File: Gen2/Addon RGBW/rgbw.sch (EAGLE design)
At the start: 33 parts, among them Q1 BUZ11, Q2 BUZ11, Q3 BUZ11, Q4 BUZ11, Q5 BUZ11, Q6 BUZ11, Q7 BUZ11, Q8 BUZ11

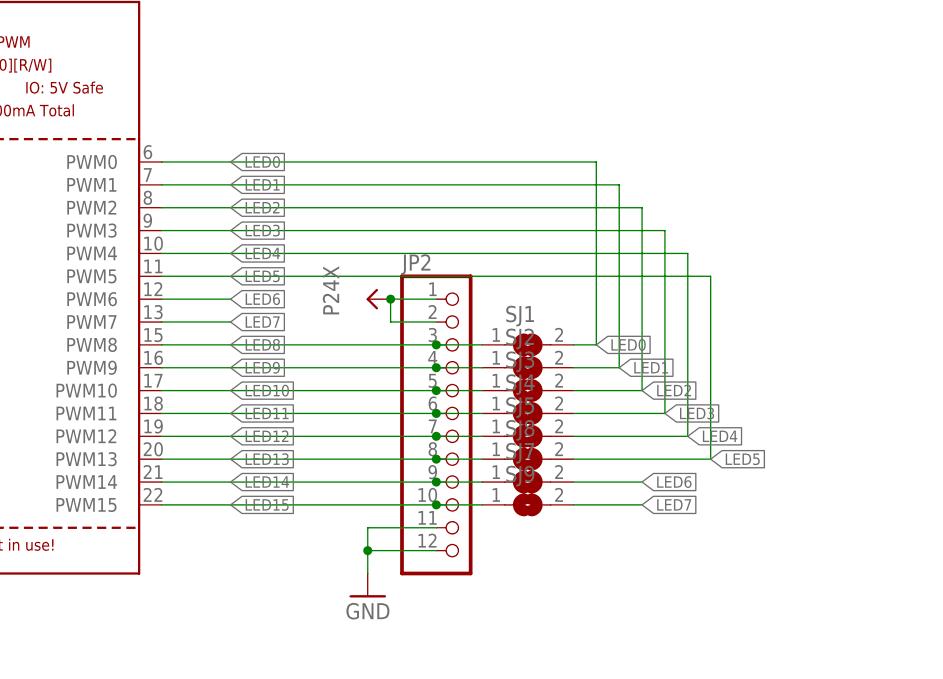
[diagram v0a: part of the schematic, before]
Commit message: ordner umsortiert und module weiter gemacht
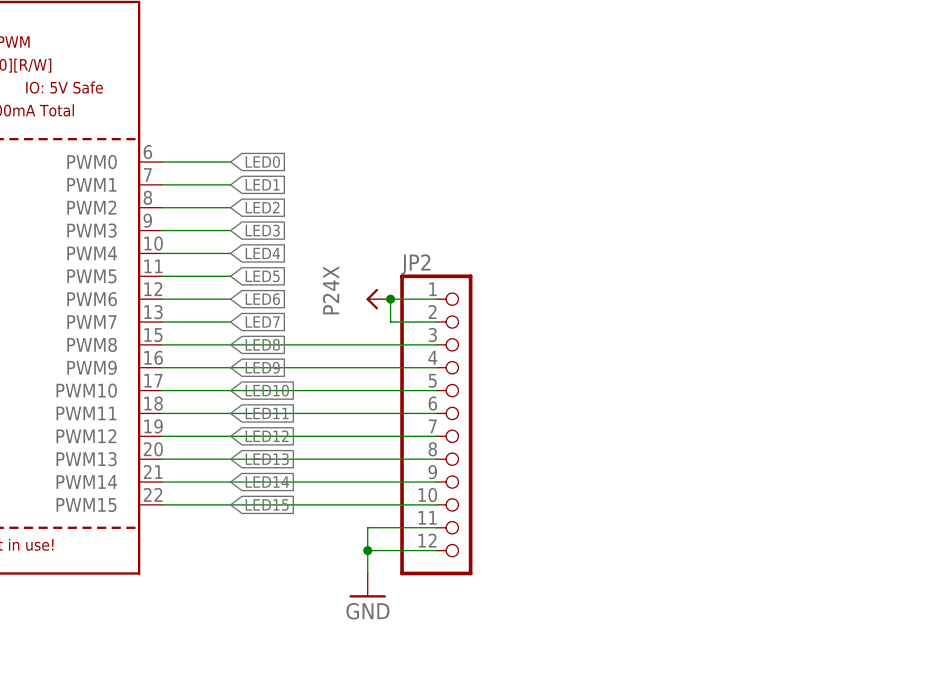
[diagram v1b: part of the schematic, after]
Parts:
- removed SJ1, SJ2, SJ3, SJ4, SJ5, SJ7, SJ8, SJ9: (no value), jumper:SJ
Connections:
- net LED0: no longer SJ1.2
- net LED1: no longer SJ2.2
- net LED10: no longer SJ3.1
- net LED11: no longer SJ4.1
- net LED12: no longer SJ5.1
- net LED13: no longer SJ8.1
- net LED14: no longer SJ7.1
- net LED15: no longer SJ9.1
- net LED2: no longer SJ3.2
- net LED3: no longer SJ4.2
- net LED4: no longer SJ5.2
- net LED5: no longer SJ8.2
- net LED6: no longer SJ7.2
- net LED7: no longer SJ9.2
- net LED8: no longer SJ1.1
- net LED9: no longer SJ2.1
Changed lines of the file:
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@@
 <part name="SUPPLY9" library="schlager_supply" deviceset="P24X" device=""/>
 <part name="GND12" library="supply1" deviceset="GND" device=""/>
-<part name="SJ1" library="jumper" deviceset="SJ" device=""/>
-<part name="SJ2" library="jumper" deviceset="SJ" device=""/>
-<part name="SJ3" library="jumper" deviceset="SJ" device=""/>
-<part name="SJ4" library="jumper" deviceset="SJ" device=""/>
-<part name="SJ5" library="jumper" deviceset="SJ" device=""/>
-<part name="SJ7" library="jumper" deviceset="SJ" device=""/>
-<part name="SJ8" library="jumper" deviceset="SJ" device=""/>
-<part name="SJ9" library="jumper" deviceset="SJ" device=""/>
 </parts>
 <sheets>
@@
 <instance part="SUPPLY9" gate="G$1" x="152.4" y="114.3" rot="R90"/>
 <instance part="GND12" gate="1" x="152.4" y="81.28" rot="MR0"/>
-<instance part="SJ1" gate="1" x="170.18" y="109.22"/>
-<instance part="SJ2" gate="1" x="170.18" y="106.68"/>
-<instance part="SJ3" gate="1" x="170.18" y="104.14"/>
-<instance part="SJ4" gate="1" x="170.18" y="101.6"/>
-<instance part="SJ5" gate="1" x="170.18" y="99.06"/>
-<instance part="SJ7" gate="1" x="170.18" y="93.98"/>
-<instance part="SJ8" gate="1" x="170.18" y="96.52"/>
-<instance part="SJ9" gate="1" x="170.18" y="91.44"/>
 </instances>
 <busses>
@@
 <pinref part="U1" gate="G$1" pin="PWM4"/>
 <label x="137.16" y="119.38" size="1.27" layer="95" xref="yes"/>
-<wire x1="129.54" y1="119.38" x2="187.96" y2="119.38" width="0.1524" layer="91"/>
-<wire x1="187.96" y1="119.38" x2="187.96" y2="99.06" width="0.1524" layer="91"/>
-<pinref part="SJ5" gate="1" pin="2"/>
-<wire x1="187.96" y1="99.06" x2="175.26" y2="99.06" width="0.1524" layer="91"/>
-<label x="187.96" y="99.06" size="1.27" layer="95" xref="yes"/>
+<wire x1="129.54" y1="119.38" x2="137.16" y2="119.38" width="0.1524" layer="91"/>
 </segment>
 </net>
@@
 <pinref part="U1" gate="G$1" pin="PWM5"/>
 <label x="137.16" y="116.84" size="1.27" layer="95" xref="yes"/>
-<wire x1="129.54" y1="116.84" x2="190.5" y2="116.84" width="0.1524" layer="91"/>
-<wire x1="190.5" y1="116.84" x2="190.5" y2="96.52" width="0.1524" layer="91"/>
-<pinref part="SJ8" gate="1" pin="2"/>
-<wire x1="190.5" y1="96.52" x2="175.26" y2="96.52" width="0.1524" layer="91"/>
-<label x="190.5" y="96.52" size="1.27" layer="95" xref="yes"/>
+<wire x1="129.54" y1="116.84" x2="137.16" y2="116.84" width="0.1524" layer="91"/>
 </segment>
 </net>
@@
 <label x="137.16" y="114.3" size="1.27" layer="95" xref="yes"/>
 </segment>
-<segment>
-<pinref part="SJ7" gate="1" pin="2"/>
-<wire x1="175.26" y1="93.98" x2="182.88" y2="93.98" width="0.1524" layer="91"/>
-<label x="182.88" y="93.98" size="1.27" layer="95" xref="yes"/>
-</segment>
 </net>
 <net name="LED7" class="0">
@@
 <pinref part="U1" gate="G$1" pin="PWM7"/>
 <label x="137.16" y="111.76" size="1.27" layer="95" xref="yes"/>
-</segment>
-<segment>
-<pinref part="SJ9" gate="1" pin="2"/>
-<wire x1="182.88" y1="91.44" x2="175.26" y2="91.44" width="0.1524" layer="91"/>
-<label x="182.88" y="91.44" size="1.27" layer="95" xref="yes"/>
 </segment>
 </net>
@@
 <pinref part="U1" gate="G$1" pin="PWM0"/>
 <label x="137.16" y="129.54" size="1.27" layer="95" xref="yes"/>
-<pinref part="SJ1" gate="1" pin="2"/>
-<wire x1="175.26" y1="109.22" x2="177.8" y2="109.22" width="0.1524" layer="91"/>
-<wire x1="177.8" y1="109.22" x2="177.8" y2="129.54" width="0.1524" layer="91"/>
-<wire x1="177.8" y1="129.54" x2="129.54" y2="129.54" width="0.1524" layer="91"/>
-<label x="177.8" y="109.22" size="1.27" layer="95" xref="yes"/>
+<wire x1="137.16" y1="129.54" x2="129.54" y2="129.54" width="0.1524" layer="91"/>
 </segment>
 </net>
@@
 <pinref part="U1" gate="G$1" pin="PWM1"/>
 <label x="137.16" y="127" size="1.27" layer="95" xref="yes"/>
-<wire x1="129.54" y1="127" x2="180.34" y2="127" width="0.1524" layer="91"/>
-<wire x1="180.34" y1="127" x2="180.34" y2="106.68" width="0.1524" layer="91"/>
-<pinref part="SJ2" gate="1" pin="2"/>
-<wire x1="180.34" y1="106.68" x2="175.26" y2="106.68" width="0.1524" layer="91"/>
-<label x="180.34" y="106.68" size="1.27" layer="95" xref="yes"/>
+<wire x1="129.54" y1="127" x2="137.16" y2="127" width="0.1524" layer="91"/>
 </segment>
 </net>
@@
 <pinref part="U1" gate="G$1" pin="PWM2"/>
 <label x="137.16" y="124.46" size="1.27" layer="95" xref="yes"/>
-<wire x1="129.54" y1="124.46" x2="182.88" y2="124.46" width="0.1524" layer="91"/>
-<wire x1="182.88" y1="124.46" x2="182.88" y2="104.14" width="0.1524" layer="91"/>
-<pinref part="SJ3" gate="1" pin="2"/>
-<wire x1="182.88" y1="104.14" x2="175.26" y2="104.14" width="0.1524" layer="91"/>
-<label x="182.88" y="104.14" size="1.27" layer="95" xref="yes"/>
+<wire x1="129.54" y1="124.46" x2="137.16" y2="124.46" width="0.1524" layer="91"/>
 </segment>
 </net>
@@
 <pinref part="U1" gate="G$1" pin="PWM3"/>
 <label x="137.16" y="121.92" size="1.27" layer="95" xref="yes"/>
-<wire x1="129.54" y1="121.92" x2="185.42" y2="121.92" width="0.1524" layer="91"/>
-<wire x1="185.42" y1="121.92" x2="185.42" y2="101.6" width="0.1524" layer="91"/>
-<pinref part="SJ4" gate="1" pin="2"/>
-<wire x1="185.42" y1="101.6" x2="175.26" y2="101.6" width="0.1524" layer="91"/>
-<label x="185.42" y="101.6" size="1.27" layer="95" xref="yes"/>
+<wire x1="129.54" y1="121.92" x2="137.16" y2="121.92" width="0.1524" layer="91"/>
 </segment>
 </net>
@@
 <pinref part="JP2" gate="G$1" pin="3"/>
 <wire x1="160.02" y1="109.22" x2="129.54" y2="109.22" width="0.1524" layer="91"/>
-<pinref part="SJ1" gate="1" pin="1"/>
-<wire x1="160.02" y1="109.22" x2="165.1" y2="109.22" width="0.1524" layer="91"/>
-<junction x="160.02" y="109.22"/>
 </segment>
 </net>
@@
 <pinref part="JP2" gate="G$1" pin="4"/>
 <wire x1="129.54" y1="106.68" x2="160.02" y2="106.68" width="0.1524" layer="91"/>
-<pinref part="SJ2" gate="1" pin="1"/>
-<wire x1="165.1" y1="106.68" x2="160.02" y2="106.68" width="0.1524" layer="91"/>
-<junction x="160.02" y="106.68"/>
 </segment>
 </net>
@@
 <pinref part="JP2" gate="G$1" pin="6"/>
 <wire x1="129.54" y1="101.6" x2="160.02" y2="101.6" width="0.1524" layer="91"/>
-<pinref part="SJ4" gate="1" pin="1"/>
-<wire x1="165.1" y1="101.6" x2="160.02" y2="101.6" width="0.1524" layer="91"/>
-<junction x="160.02" y="101.6"/>
 </segment>
 </net>
@@
 <pinref part="JP2" gate="G$1" pin="7"/>
 <wire x1="160.02" y1="99.06" x2="129.54" y2="99.06" width="0.1524" layer="91"/>
-<pinref part="SJ5" gate="1" pin="1"/>
-<wire x1="165.1" y1="99.06" x2="160.02" y2="99.06" width="0.1524" layer="91"/>
-<junction x="160.02" y="99.06"/>
 </segment>
 </net>
@@
 <pinref part="JP2" gate="G$1" pin="8"/>
 <wire x1="129.54" y1="96.52" x2="160.02" y2="96.52" width="0.1524" layer="91"/>
-<pinref part="SJ8" gate="1" pin="1"/>
-<wire x1="160.02" y1="96.52" x2="165.1" y2="96.52" width="0.1524" layer="91"/>
-<junction x="160.02" y="96.52"/>
 </segment>
 </net>
@@
 <pinref part="JP2" gate="G$1" pin="9"/>
 <wire x1="160.02" y1="93.98" x2="129.54" y2="93.98" width="0.1524" layer="91"/>
-<pinref part="SJ7" gate="1" pin="1"/>
-<wire x1="165.1" y1="93.98" x2="160.02" y2="93.98" width="0.1524" layer="91"/>
-<junction x="160.02" y="93.98"/>
 </segment>
 </net>
@@
 <pinref part="JP2" gate="G$1" pin="10"/>
 <wire x1="129.54" y1="91.44" x2="160.02" y2="91.44" width="0.1524" layer="91"/>
-<pinref part="SJ9" gate="1" pin="1"/>
-<wire x1="165.1" y1="91.44" x2="160.02" y2="91.44" width="0.1524" layer="91"/>
-<junction x="160.02" y="91.44"/>
 </segment>
 </net>
@@
 <pinref part="JP2" gate="G$1" pin="5"/>
 <wire x1="160.02" y1="104.14" x2="129.54" y2="104.14" width="0.1524" layer="91"/>
-<pinref part="SJ3" gate="1" pin="1"/>
-<wire x1="160.02" y1="104.14" x2="165.1" y2="104.14" width="0.1524" layer="91"/>
-<junction x="160.02" y="104.14"/>
-</segment>
-</net>
+</segment>
+</net>
